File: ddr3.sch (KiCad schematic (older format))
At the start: 39 parts, among them U7 AS4C256M16D3, U8 TPS51200DRC

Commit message: Updated local libs
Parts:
- R13: footprint antmicro-footprints:0402-res -> artix-dc-scm-footprints:0402-res; symbol antmicroResistors0402:R_4k7_0402 -> artix-dc-scm:R_4k7_0402
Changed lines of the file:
@@
 $EndComp
 $Comp
-L antmicroResistors0402:R_4k7_0402 R13
+L artix-dc-scm:R_4k7_0402 R13
 U 1 1 5FF6FE54
 P 3850 6150
 F 0 "R13" V 3805 6220 60  0000 L CNN
 F 1 "R_4k7_0402" H 3850 6000 60  0001 C CNN
-F 2 "antmicro-footprints:0402-res" H 4050 6350 60  0001 L CNN
+F 2 "artix-dc-scm-footprints:0402-res" H 4050 6350 60  0001 L CNN
 F 3 "" H 3850 6150 50  0001 C CNN
 F 4 "PANASONIC_ELECTRONIC_COMPONENTS" H 4050 6550 60  0001 L CNN "Manufacturer"

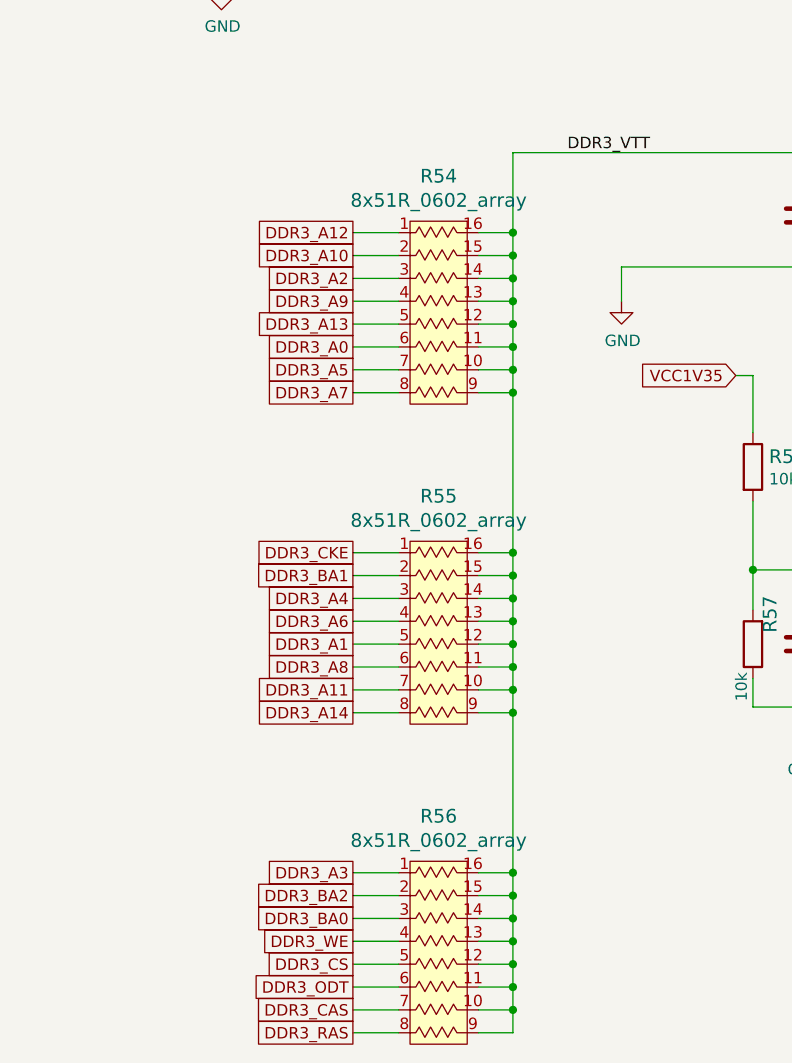
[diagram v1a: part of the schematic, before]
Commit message: Update DDR3 termination
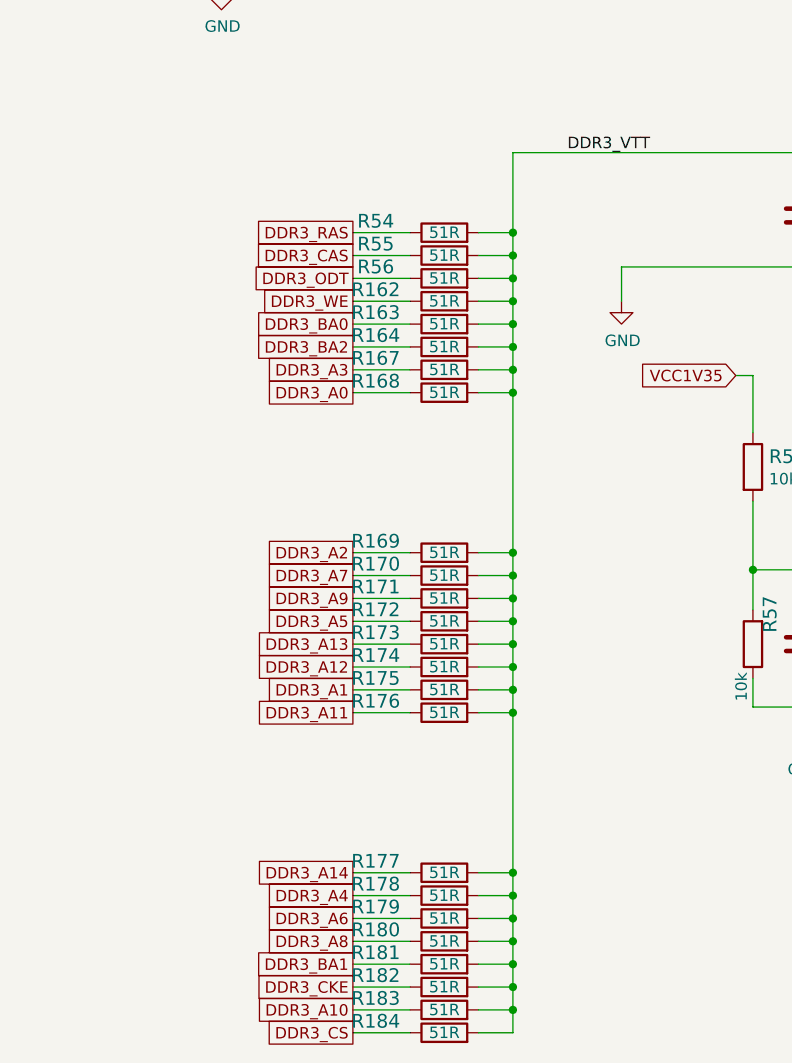
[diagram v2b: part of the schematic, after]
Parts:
- removed R54, R55, R56: 8x51R_0602_array, artix-dc-scm-footprints:R_Array_Convex_8x0602, symbol artix-dc-scm:8x51R_0602_array
- added R162, R163, R164, R167, R168, R169, R170, R171, R172, R173, R174, R175, R176, R177, R178, R179, R180, R181, R182, R183, R184, R54, R55, R56: R_51R_0402, antmicro-footprints:0402-res, symbol antmicroResistors0402:R_51R_0402
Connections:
- net DDR3_A0: now also R168.1
- net DDR3_A1: now also R175.1
- net DDR3_A10: now also R183.1
- net DDR3_A11: now also R176.1
- net DDR3_A12: now also R174.1
- net DDR3_A13: now also R173.1
- net DDR3_A14: now also R177.1
- net DDR3_A2: now also R169.1
- net DDR3_A3: now also R167.1
- net DDR3_A4: now also R178.1
- net DDR3_A5: now also R172.1
- net DDR3_A6: now also R179.1
- net DDR3_A7: now also R170.1
- net DDR3_A8: now also R180.1
- net DDR3_A9: now also R171.1
- net DDR3_BA0: now also R163.1
- net DDR3_BA1: now also R181.1
- net DDR3_BA2: now also R164.1
- net DDR3_CAS: now also R55.1
- net DDR3_CKE: now also R182.1
- net DDR3_CS: now also R184.1
- net DDR3_ODT: now also R56.1
- net DDR3_RAS: now also R54.1
- net DDR3_VTT: now also R162.2, R163.2, R164.2, R167.2, R168.2, R169.2, R170.2, R171.2, R172.2, R173.2, R174.2, R175.2, R176.2, R177.2, R178.2, R179.2, R180.2, R181.2, R182.2, R183.2, R184.2, R54.2, R55.2, R56.2
- net DDR3_WE: now also R162.1
